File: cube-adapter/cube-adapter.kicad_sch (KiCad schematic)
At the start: 44 parts, among them J1 Conn_01x02, J10 Conn_01x02, J11 Conn_01x03, J12 Conn_01x03, J13 Conn_01x03, J14 Conn_01x03, J15 Conn_01x03, J16 Conn_01x03, J17 Conn_01x03, J18 Conn_01x03, J19 Conn_01x03, J2 Conn_01x02, J20 Conn_01x03, J21 Conn_01x03, J22 Conn_01x03, J23 Conn_01x06, J24 Conn_01x06, J25 Conn_01x04, J26 Conn_01x04, J27 Conn_01x05, J28 Conn_01x05, J29 Conn_01x05, J3 Conn_01x02, J30 Conn_01x04, J31 Conn_01x04, J32 Conn_01x04, J33 Conn_01x03, J34 Conn_01x03, J35 Conn_01x03, J36 Conn_01x02, J37 Conn_01x02, J38 Conn_01x02, J4 Conn_01x02, J5 Conn_01x02, J6 Conn_01x02, J7 Conn_01x02, J8 Conn_01x02, J9 Conn_01x02, U1 MEGA_PRO_EMBED_CH340G___ATMEG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

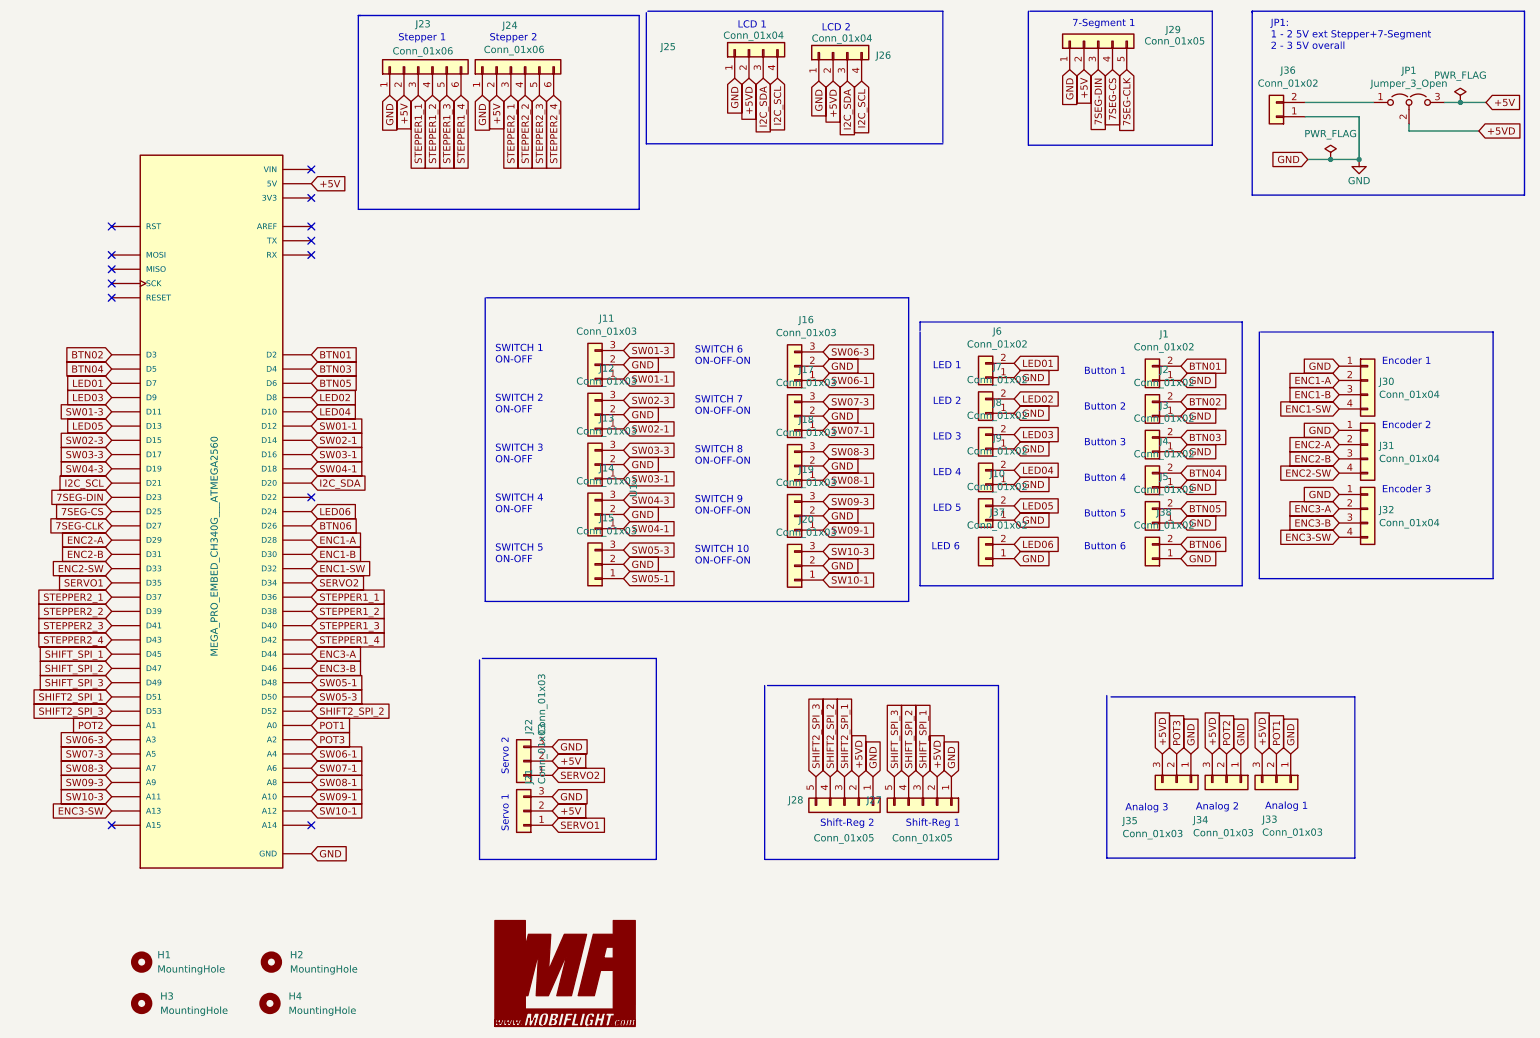
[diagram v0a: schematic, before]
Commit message: v2.0 of cube adapter
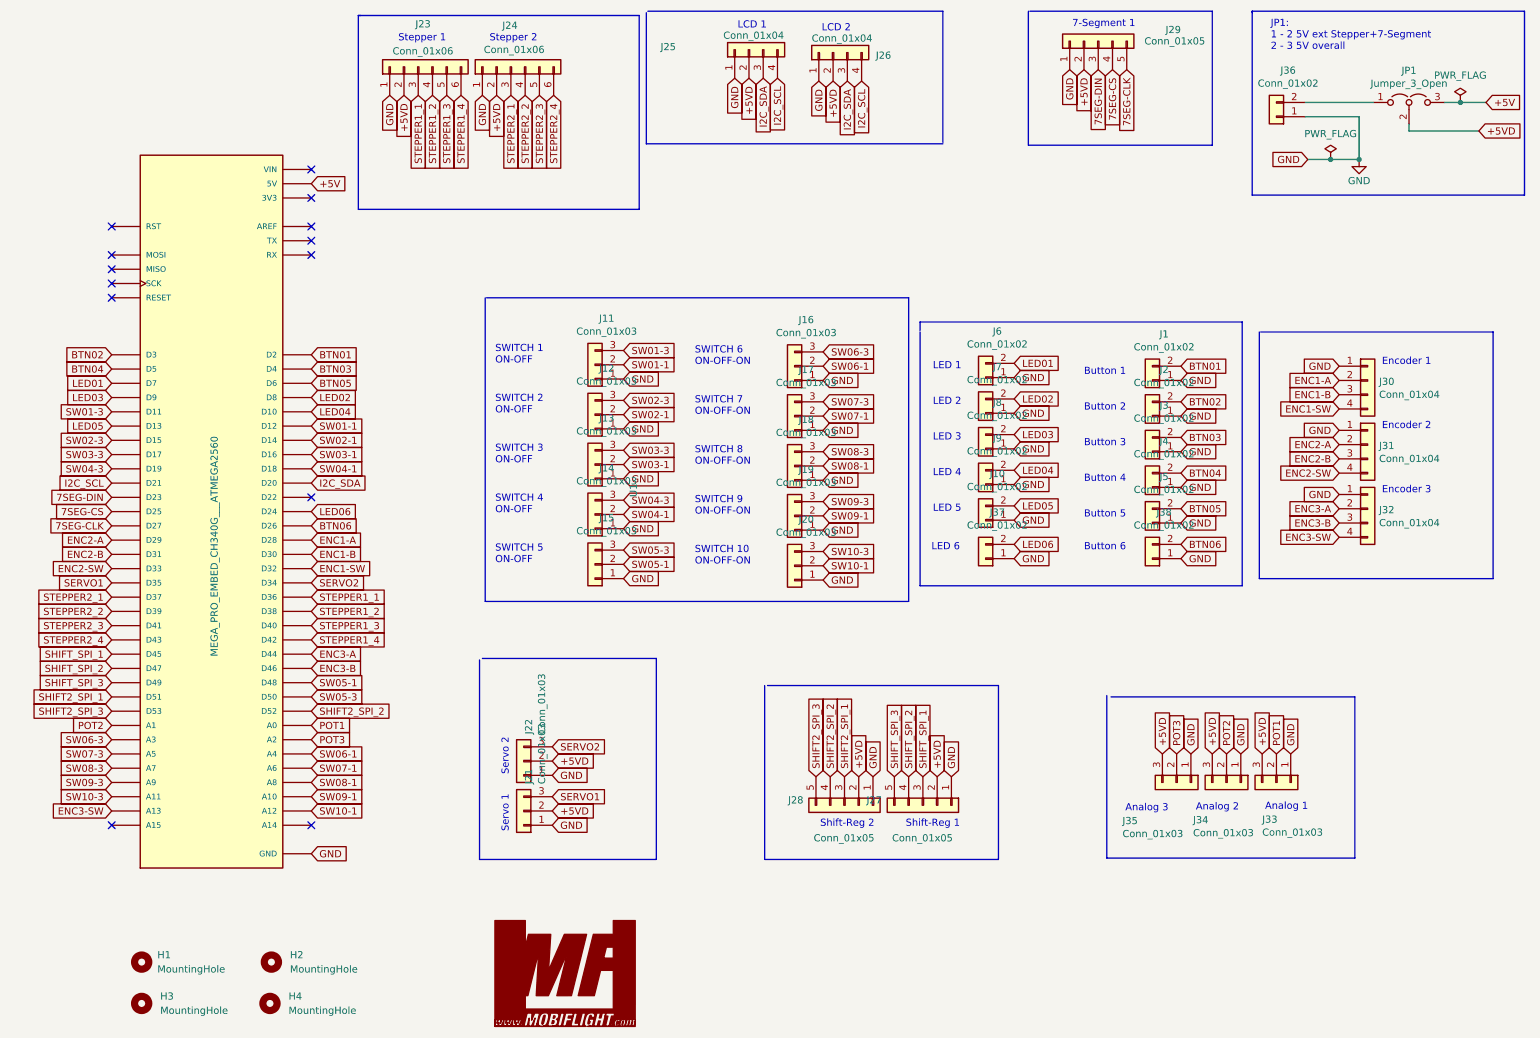
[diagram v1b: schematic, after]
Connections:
- net +5V: no longer J21.2 (Pin_2), J22.2 (Pin_2), J23.2 (Pin_2), J24.2 (Pin_2), J29.2 (Pin_2)
- net +5VD: now also J21.2 (Pin_2), J22.2 (Pin_2), J23.2 (Pin_2), J24.2 (Pin_2), J29.2 (Pin_2)
- net GND: now also J11.1 (Pin_1), J12.1 (Pin_1), J13.1 (Pin_1), J14.1 (Pin_1), J15.1 (Pin_1), J16.1 (Pin_1), J17.1 (Pin_1), J18.1 (Pin_1), J19.1 (Pin_1), J20.1 (Pin_1), J21.1 (Pin_1), J22.1 (Pin_1); no longer J11.2 (Pin_2), J12.2 (Pin_2), J13.2 (Pin_2), J14.2 (Pin_2), J15.2 (Pin_2), J16.2 (Pin_2), J17.2 (Pin_2), J18.2 (Pin_2), J19.2 (Pin_2), J20.2 (Pin_2), J21.3 (Pin_3), J22.3 (Pin_3)
- net SERVO1: now also J21.3 (Pin_3); no longer J21.1 (Pin_1)
- net SERVO2: now also J22.3 (Pin_3); no longer J22.1 (Pin_1)
- net SW01-1: now also J11.2 (Pin_2); no longer J11.1 (Pin_1)
- net SW02-1: now also J12.2 (Pin_2); no longer J12.1 (Pin_1)
- net SW03-1: now also J13.2 (Pin_2); no longer J13.1 (Pin_1)
- net SW04-1: now also J14.2 (Pin_2); no longer J14.1 (Pin_1)
- net SW05-1: now also J15.2 (Pin_2); no longer J15.1 (Pin_1)
- net SW06-1: now also J16.2 (Pin_2); no longer J16.1 (Pin_1)
- net SW07-1: now also J17.2 (Pin_2); no longer J17.1 (Pin_1)
- net SW08-1: now also J18.2 (Pin_2); no longer J18.1 (Pin_1)
- net SW09-1: now also J19.2 (Pin_2); no longer J19.1 (Pin_1)
- net SW10-1: now also J20.2 (Pin_2); no longer J20.1 (Pin_1)
